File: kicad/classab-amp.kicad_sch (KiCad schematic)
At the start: 64 parts, among them J1 SPEAKER, J3 INPUT, Q1 2N5551, Q10 IRFP9240, Q11 2N5551, Q12 2N5551, Q15 2N5551, Q16 2N5401, Q2 2N5551, Q3 2N5401, Q4 2N5401, Q6 BD140, Q7 BD139, Q8 BD139, Q9 IRFP240

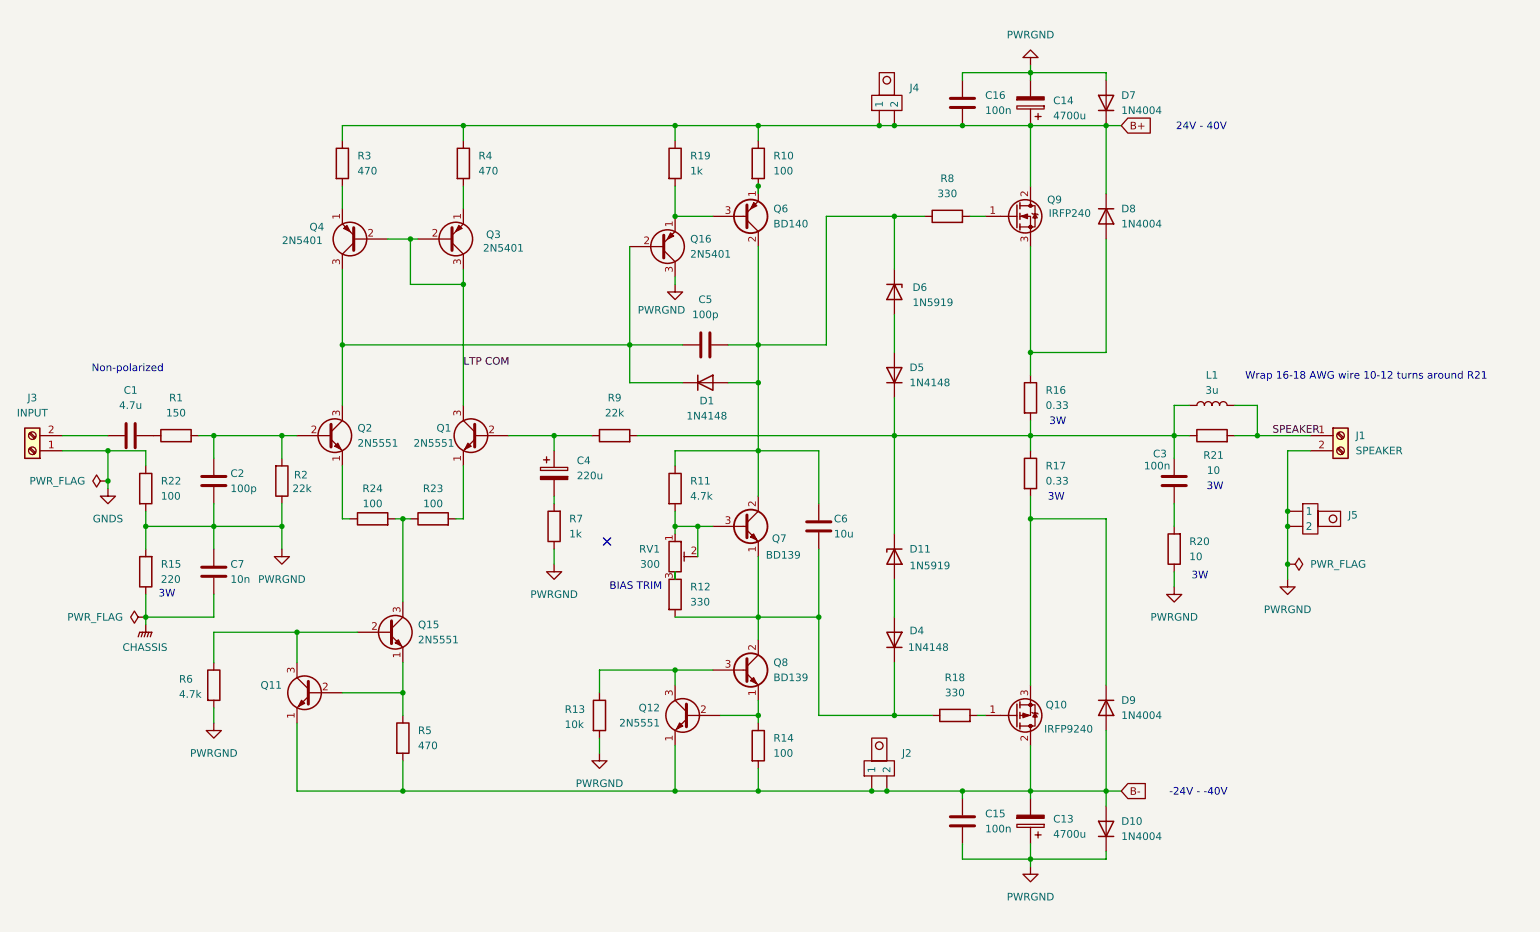
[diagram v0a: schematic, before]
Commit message: 2.0 stuff
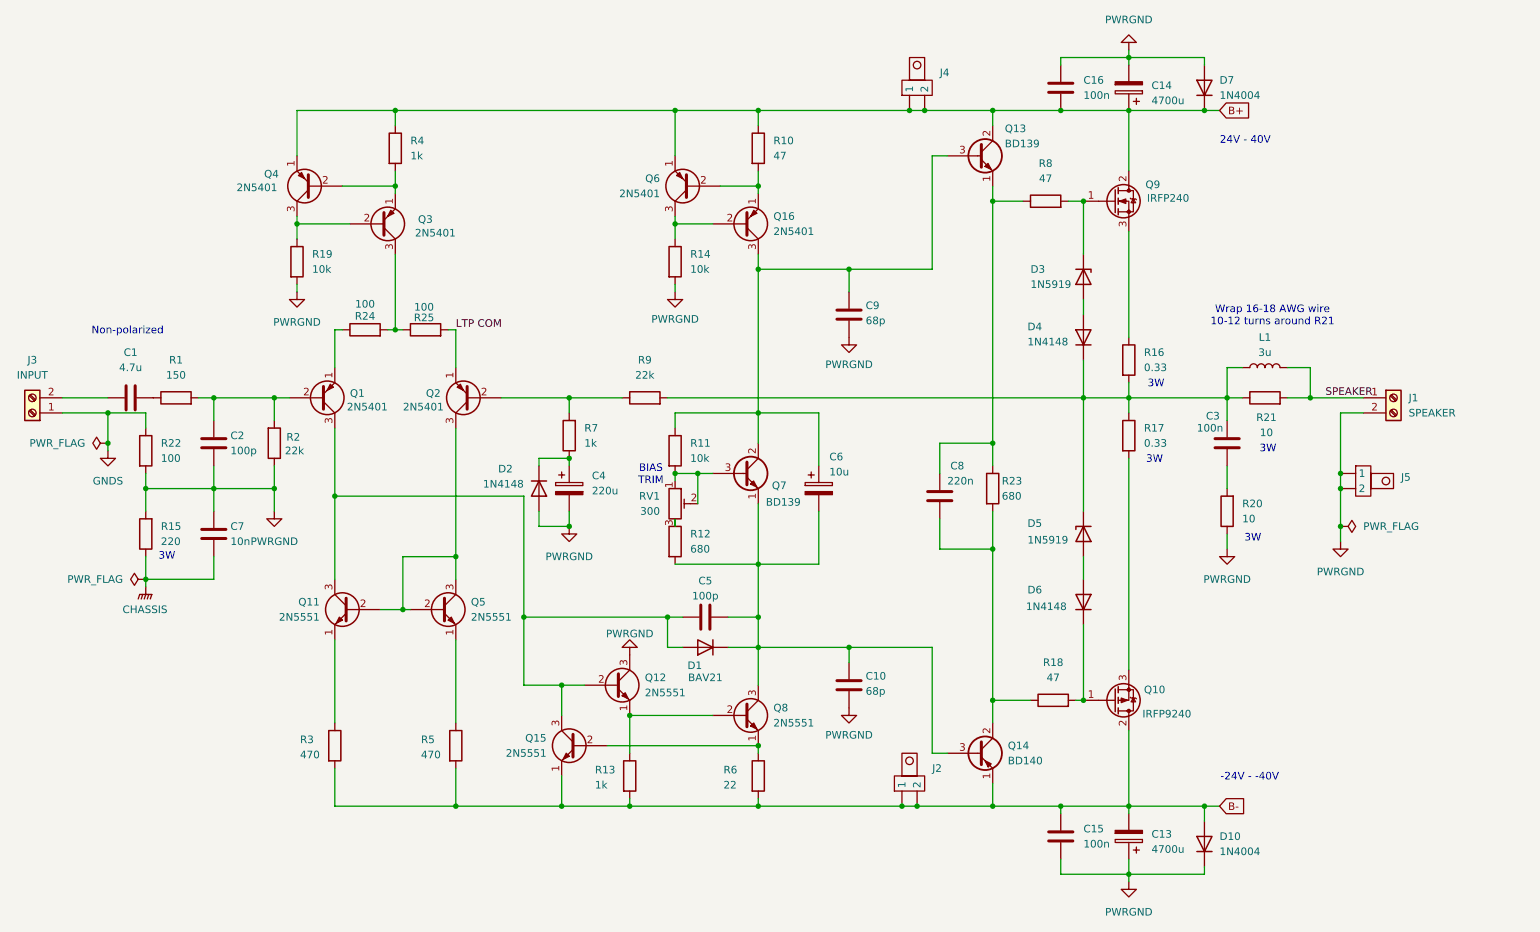
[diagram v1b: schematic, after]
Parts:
- removed C6: 10u, Capacitor_THT:CP_Radial_D4.0mm_P2.00mm, symbol Device:C
- removed D1, D5: 1N4148, Diode_THT:D_DO-35_SOD27_P7.62mm_Horizontal, symbol Diode:1N4148
- removed D11, D6: 1N5919, Diode_THT:D_DO-41_SOD81_P10.16mm_Horizontal, symbol Device:D_Zener
- removed D8, D9: 1N4004, Diode_THT:D_DO-41_SOD81_P10.16mm_Horizontal, symbol Diode:1N4004
- removed Q1, Q2: 2N5551, Package_TO_SOT_THT:TO-92_Wide, symbol Custom:2N5551
- removed Q6: BD140, Package_TO_SOT_THT:TO-126-3_Vertical, symbol Transistor_BJT:BD140
- removed Q8: BD139, Package_TO_SOT_THT:TO-126-3_Vertical, symbol Transistor_BJT:BD139
- added C10, C9: 68p, Capacitor_THT:CP_Radial_D4.0mm_P2.00mm, symbol Device:C
- added C6: 10u, symbol Device:C_Polarized
- added C8: 220n, Capacitor_THT:CP_Radial_D4.0mm_P2.00mm, symbol Device:C
- added D1: BAV21, Diode_THT:D_DO-35_SOD27_P7.62mm_Horizontal, symbol Diode:BAV21
- added D2, D6: 1N4148, Diode_THT:D_DO-35_SOD27_P7.62mm_Horizontal, symbol Diode:1N4148
- added D3, D5: 1N5919, Diode_THT:D_DO-41_SOD81_P10.16mm_Horizontal, symbol Device:D_Zener
- added Q1, Q2, Q6: 2N5401, Package_TO_SOT_THT:TO-92_Wide, symbol Custom:2N5401
- added Q13: BD139, Package_TO_SOT_THT:TO-126-3_Vertical, symbol Transistor_BJT:BD139
- added Q14: BD140, Package_TO_SOT_THT:TO-126-3_Vertical, symbol Transistor_BJT:BD140
- added Q5, Q8: 2N5551, Package_TO_SOT_THT:TO-92_Wide, symbol Custom:2N5551
- added R25: 100, Resistor_THT:R_Axial_DIN0207_L6.3mm_D2.5mm_P2.54mm_Vertical, symbol Device:R
- C4: footprint Capacitor_THT:CP_Radial_D8.0mm_P5.00mm -> (none)
- R10: value 100 -> 47
- R11: value 4.7k -> 10k
- R12: value 330 -> 680
- R13: value 10k -> 1k
- R14: value 100 -> 10k; footprint Resistor_THT:R_Axial_DIN0204_L3.6mm_D1.6mm_P7.62mm_Horizontal -> Resistor_THT:R_Axial_DIN0207_L6.3mm_D2.5mm_P2.54mm_Vertical
- R18, R8: value 330 -> 47
- R19: value 1k -> 10k
- R23: value 100 -> 680
- R4: value 470 -> 1k
- R6: value 4.7k -> 22
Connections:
- net B+: now also Q4.1 (E), Q13.2 (C), Q6.1 (E); no longer R19.1, R3.1
- net B-: now also Q15.1 (E), R13.2, R3.2, R6.2, Q14.1 (E); no longer Q11.1 (E), Q12.1 (E), R14.2
- net LTP COM: now also Q2.1 (E), R25.2; no longer Q3.2 (B), Q3.3 (C), Q4.2 (B)
- net PWRGND: now also C4.2, Q12.3 (C), R14.2, R19.2, C10.2, C9.2, D2.2 (A); no longer Q16.3 (C), R13.2, R6.2, R7.1
- net at C3.1, L1.1, R16.2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: now also D4.1 (K), D5.1 (K)
- net at Q12.2 (B): now also C5.1, Q11.3 (C), Q15.3 (C), D1.2 (A), Q1.3 (C); no longer R14.1
- net at R13.1: now also Q12.1 (E), Q8.2 (B); no longer Q12.3 (C)
- net at Q15.2 (B), R6.1: now also Q8.1 (E); no longer Q11.3 (C)
- net at R10.2: now also Q16.1 (E), Q6.2 (B)
- net at Q7.2 (C), R11.1: now also Q16.3 (C), C6.1, C9.1, Q13.3 (B); no longer C5.2, R8.1
- net at R24.1: now also Q1.1 (E)
- net at Q9.1 (G), R8.2: now also D3.1 (K)
- net at C2.1, R1.2, R2.2: now also Q1.2 (B)
- net at R9.1: now also R7.2, Q2.2 (B); no longer C4.1
- net at D4.2 (A): now also D3.2 (A)
- net at Q10.1 (G), R18.2: now also D6.1 (K)
- net at Q7.1 (E), R12.2: now also C5.2, C10.1, C6.2, D1.1 (K), Q14.3 (B), Q8.3 (C); no longer D4.1 (K), R18.1
- net at R23.2: now also R18.1, C8.2, Q14.2 (C)
- net at Q3.1 (E), R4.2: now also Q4.2 (B)
- new net: Q3.2 (B), Q4.3 (C), R19.1
- new net: Q16.2 (B), Q6.3 (C), R14.1
- new net: D5.2 (A), D6.2 (A)
- new net: C8.1, Q13.1 (E), R23.1, R8.1
- new net: Q5.1 (E), R5.1
- new net: Q11.2 (B), Q2.3 (C), Q5.2 (B), Q5.3 (C)
- new net: C4.1, D2.1 (K), R7.1
- new net: Q11.1 (E), R3.1
- new net: Q3.3 (C), R24.2, R25.1
- no-connect marks 1 -> 0
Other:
- moved on the sheet: C1, C13, C14, C15, C16, C2, C3, C7, D10, D7, J1, J2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
